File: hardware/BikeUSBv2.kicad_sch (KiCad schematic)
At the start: 55 parts, among them J1 TYPE-C-31-M-16, J2 JST S2B-EH(LF)(SN), Q1 2SB772SQ, SW1 1TS002E-2500-2501-CT, SW2 1TS002E-2500-2501-CT, U1 TPS63070, U2 ATtiny1616-M, U3 FUSB302B10MPX, U4 HT7550, U5 TL431AIDBZR

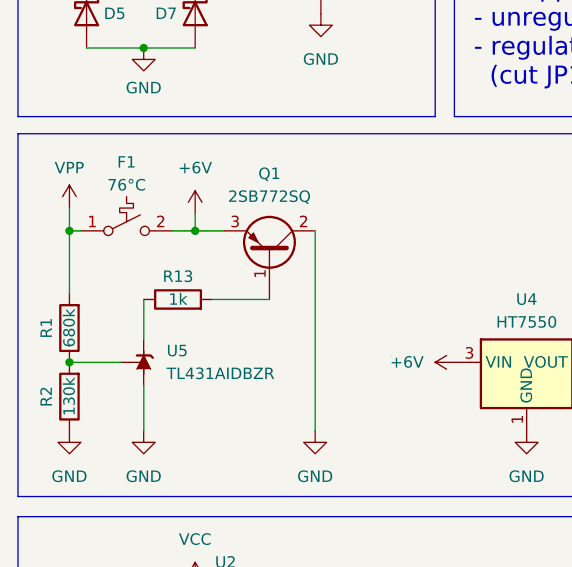
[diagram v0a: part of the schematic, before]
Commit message: [PCB] slight sch change
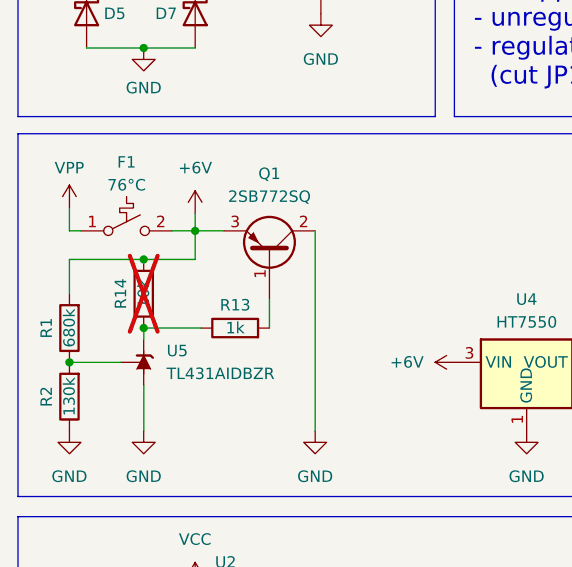
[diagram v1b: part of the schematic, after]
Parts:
- added R14: 10k, Resistor_SMD:R_0805_2012Metric_Pad1.20x1.40mm_HandSolder, symbol Device:R
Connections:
- net +6V: now also R1.2, R14.2
- net VPP: no longer R1.2
- net at R13.1, U5.1 (K): now also R14.1
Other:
- moved on the sheet: R13
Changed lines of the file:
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@@
   (junction (at 161.925 27.305) (diameter 0) (color 0 0 0 0)
   )
+  (junction (at 30.48 73.66) (diameter 0) (color 0 0 0 0)
+  )
   (junction (at 142.24 57.15) (diameter 0) (color 0 0 0 0)
   )
@@
   (junction (at 151.765 27.305) (diameter 0) (color 0 0 0 0)
   )
+  (junction (at 30.48 81.28) (diameter 0) (color 0 0 0 0)
+  )
   (junction (at 71.12 120.015) (diameter 0) (color 0 0 0 0)
   )
@@
   (junction (at 151.765 34.925) (diameter 0) (color 0 0 0 0)
   )
-  (junction (at 22.225 70.485) (diameter 0) (color 0 0 0 0)
-  )
   (junction (at 142.24 27.305) (diameter 0) (color 0 0 0 0)
   )
@@
     (stroke (width 0) (type default))
   )
+  (wire (pts (xy 36.195 70.485) (xy 36.195 73.66))
+    (stroke (width 0) (type default))
+  )
   (wire (pts (xy 156.21 127) (xy 160.655 127))
     (stroke (width 0) (type default))
@@
     (stroke (width 0) (type default))
   )
-  (wire (pts (xy 51.435 137.795) (xy 56.515 137.795))
+  (wire (pts (xy 44.45 81.28) (xy 44.45 78.105))
     (stroke (width 0) (type default))
   )
-  (wire (pts (xy 30.48 82.55) (xy 30.48 78.105))
+  (wire (pts (xy 51.435 137.795) (xy 56.515 137.795))
     (stroke (width 0) (type default))
   )
@@
     (stroke (width 0) (type default))
   )
+  (wire (pts (xy 30.48 81.28) (xy 30.48 82.55))
+    (stroke (width 0) (type default))
+  )
   (wire (pts (xy 146.05 114.3) (xy 156.21 114.3))
     (stroke (width 0) (type default))
@@
     (stroke (width 0) (type default))
   )
+  (wire (pts (xy 22.225 77.47) (xy 22.225 73.66))
+    (stroke (width 0) (type default))
+  )
   (wire (pts (xy 89.535 150.495) (xy 92.71 150.495))
     (stroke (width 0) (type default))
@@
     (stroke (width 0) (type default))
   )
-  (wire (pts (xy 22.225 70.485) (xy 22.225 77.47))
+  (wire (pts (xy 36.83 81.28) (xy 30.48 81.28))
     (stroke (width 0) (type default))
   )
@@
     (stroke (width 0) (type default))
   )
+  (wire (pts (xy 30.48 73.66) (xy 36.195 73.66))
+    (stroke (width 0) (type default))
+  )
   (wire (pts (xy 154.305 71.12) (xy 158.115 71.12))
     (stroke (width 0) (type default))
@@
     (stroke (width 0) (type default))
   )
+  (wire (pts (xy 22.225 73.66) (xy 30.48 73.66))
+    (stroke (width 0) (type default))
+  )
   (wire (pts (xy 156.21 83.82) (xy 158.115 83.82))
     (stroke (width 0) (type default))
@@
     (stroke (width 0) (type default))
   )
-  (wire (pts (xy 38.1 78.105) (xy 44.45 78.105))
-    (stroke (width 0) (type default))
-  )
   (wire (pts (xy 24.13 34.925) (xy 30.48 34.925))
     (stroke (width 0) (type default))
@@
     )
   )
-  (symbol (lib_id "Device:R") (at 34.29 78.105 90) (unit 1)
+  (symbol (lib_id "Device:R") (at 40.64 81.28 90) (unit 1)
     (in_bom yes) (on_board yes) (dnp no)
-    (property "Reference" "R13" (at 34.29 75.565 90)
+    (property "Reference" "R13" (at 40.64 78.74 90)
       (effects (font (size 1.27 1.27)))
     )
-    (property "Value" "1k" (at 34.29 78.105 90)
+    (property "Value" "1k" (at 40.64 81.28 90)
       (effects (font (size 1.27 1.27)))
     )
-    (property "Footprint" "Resistor_SMD:R_0805_2012Metric_Pad1.20x1.40mm_HandSolder" (at 34.29 79.883 90)
+    (property "Footprint" "Resistor_SMD:R_0805_2012Metric_Pad1.20x1.40mm_HandSolder" (at 40.64 83.058 90)
       (effects (font (size 1.27 1.27)) hide)
     )
-    (property "Datasheet" "~" (at 34.29 78.105 0)
+    (property "Datasheet" "~" (at 40.64 81.28 0)
       (effects (font (size 1.27 1.27)) hide)
     )
-    (property "LCSC" "C110774" (at 34.29 75.565 0)
+    (property "LCSC" "C110774" (at 40.64 78.74 0)
       (effects (font (size 1.27 1.27)) hide)
     )
@@
         )
       )
+    )
+  )
+  (symbol (lib_id "Device:R") (at 30.48 77.47 180) (unit 1)
+    (in_bom yes) (on_board no) (dnp yes)
+    (property "Reference" "R14" (at 27.94 77.47 90)
+      (effects (font (size 1.27 1.27)))
+    )
+    (property "Value" "10k" (at 30.48 77.47 90)
+      (effects (font (size 1.27 1.27)))
+    )
+    (property "Footprint" "Resistor_SMD:R_0805_2012Metric_Pad1.20x1.40mm_HandSolder" (at 32.258 77.47 90)
+      (effects (font (size 1.27 1.27)) hide)
+    )
+    (property "Datasheet" "~" (at 30.48 77.47 0)
+      (effects (font (size 1.27 1.27)) hide)
+    )
+    (property "LCSC" "C217770" (at 27.94 77.47 0)
+      (effects (font (size 1.27 1.27)) hide)
+    )
+    (property "Sim.Enable" "0" (at 30.48 77.47 0)
+      (effects (font (size 1.27 1.27)) hide)
+    )
+    (pin "1")
+    (pin "2")
+    (instances
+      (project "BikeUSBv2"
+        (path "/b4aff538-5116-4944-9d24-c26a88d7dfe8"
+          (reference "R14") (unit 1)
+        )
+      )
